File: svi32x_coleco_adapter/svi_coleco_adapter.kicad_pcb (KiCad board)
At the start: 2 copper layers, 212 x 94 mm, 62 parts, among them J1 Conn_01x09, J2 Conn_01x09, J3 COLECO cartridge slot, J4 SVI external bus connector, T1 NPN_BCE_9014B, T2 NPN_BCE_9014B, U1 74LS244, U10 27C64, U11 L79L05, U2 74LS244, U3 74LS32, U4 74LS00, U5 74LS00, U6 74LS138, U7 74LS138, U8 LM741, U9 SN76489

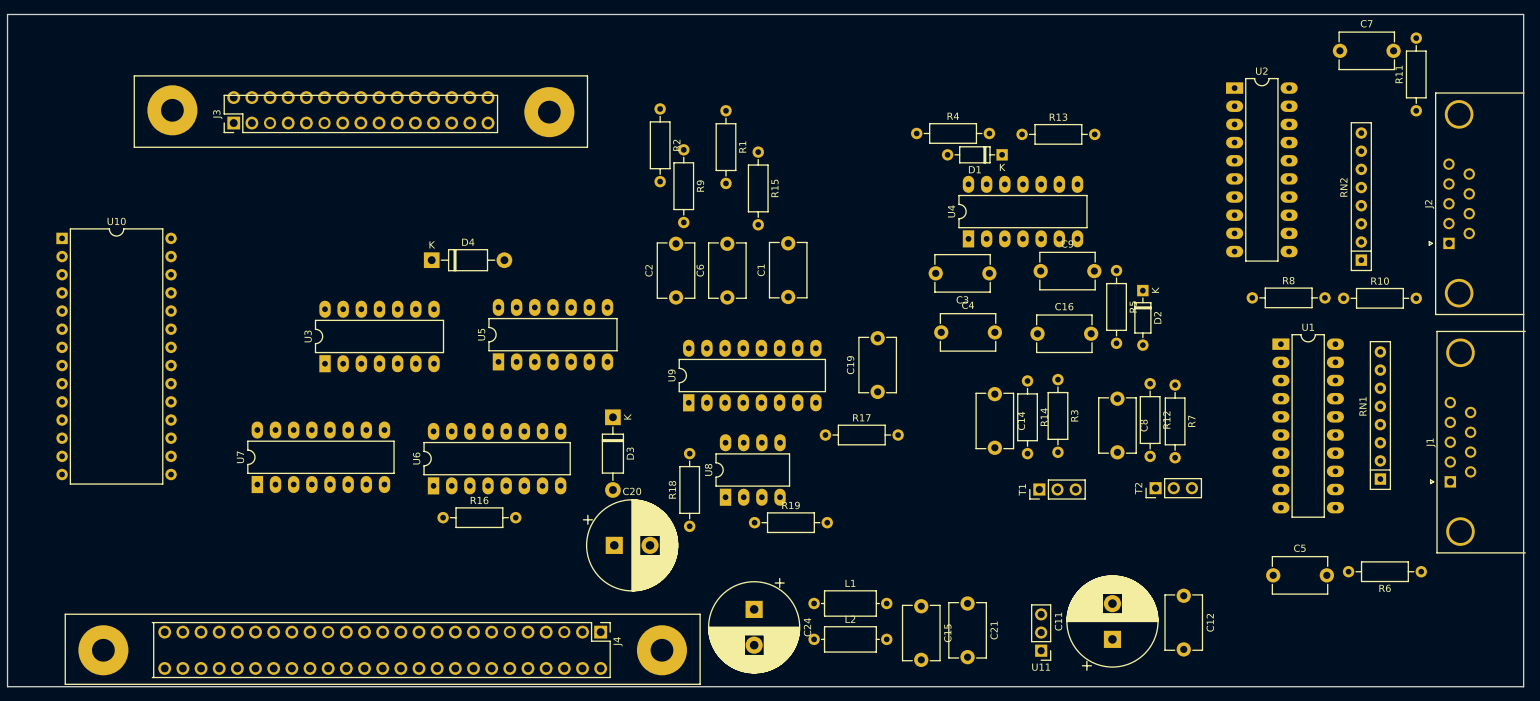
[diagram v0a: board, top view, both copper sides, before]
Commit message: Add files via upload
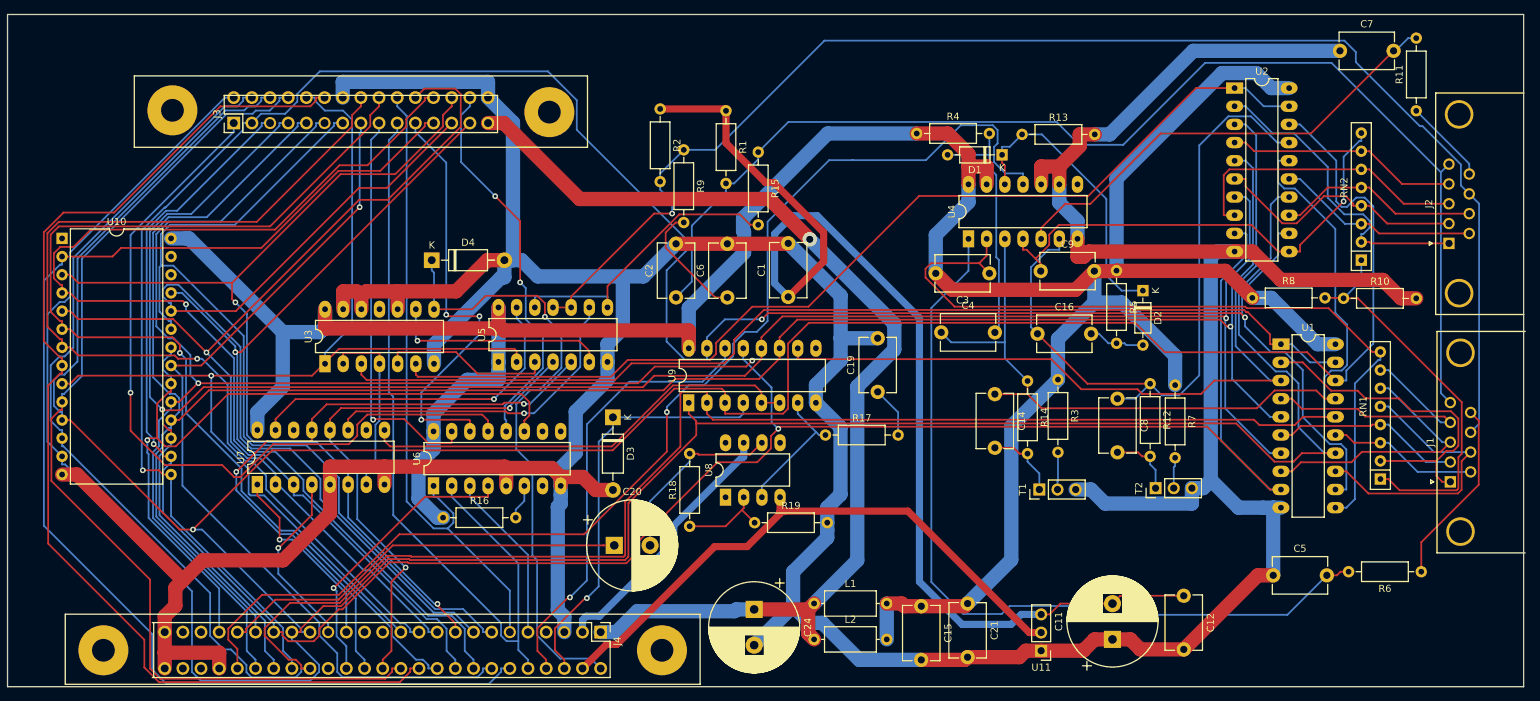
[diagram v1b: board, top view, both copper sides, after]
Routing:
- net GND: track 0.00 -> 662.8 mm
- net +5V: track 0.00 -> 420.1 mm
- net D1: track 0.00 -> 348.3 mm
- net D2: track 0.00 -> 343.8 mm
- net D0: track 0.00 -> 342.2 mm, vias 0 -> 1
- net D3: track 0.00 -> 321.8 mm, vias 0 -> 3
- net D4: track 0.00 -> 305.8 mm, vias 0 -> 2
- net D7: track 0.00 -> 304.5 mm, vias 0 -> 2
- net D5: track 0.00 -> 294.9 mm, vias 0 -> 2
- net D6: track 0.00 -> 292.1 mm, vias 0 -> 1
- net COL_JOY8: track 0.00 -> 195.9 mm, vias 0 -> 1
- net A12: track 0.00 -> 177.2 mm
- net COL_JOY5: track 0.00 -> 169.7 mm
- net _INT: track 0.00 -> 166.9 mm, vias 0 -> 1
- net A1: track 0.00 -> 159.0 mm, vias 0 -> 1
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
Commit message: Add files via upload
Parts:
- added C30: 100nf, Capacitor_THT:C_Disc_D7.0mm_W2.5mm_P5.00mm, F.Cu at (174.6, 36.1)
- added C31: 100nf, Capacitor_THT:C_Disc_D7.0mm_W2.5mm_P5.00mm, F.Cu at (196.5, 35.9)
- added C32: 100nf, Capacitor_THT:C_Disc_D7.0mm_W2.5mm_P5.00mm, F.Cu at (209.9, 91.8)
- added C33: 100nf, Capacitor_THT:C_Disc_D7.0mm_W2.5mm_P5.00mm, F.Cu at (229.2, 91.4)
- added C34: 100nf, Capacitor_THT:C_Disc_D7.0mm_W2.5mm_P5.00mm, F.Cu at (232.7, 34.7)
- added C35: 100nf, Capacitor_THT:C_Disc_D7.0mm_W2.5mm_P5.00mm, F.Cu at (256.6, 45.8)
- added C36: 100nf, Capacitor_THT:C_Disc_D7.0mm_W2.5mm_P5.00mm, F.Cu at (252.6, 115.3)
- added C37: 100nf, Capacitor_THT:C_Disc_D7.0mm_W2.5mm_P5.00mm, F.Cu at (79.6, 91.8)
- C1, C12, C14, C15, C16, C19, C2, C21, C3, C4, C5, C6, C7, C8, C9: footprint Capacitor_THT:C_Disc_D7.5mm_W5.0mm_P7.50mm -> Capacitor_THT:C_Disc_D7.0mm_W2.5mm_P5.00mm
- C20: footprint Capacitor_THT:CP_Radial_D12.5mm_P5.00mm -> Capacitor_THT:CP_Radial_D8.0mm_P5.00mm
- R12, R14: value 22R -> 22K
- moved R9 151.3 mm to (291.5, 77.7), turned to 180 degrees
- moved R2 145.0 mm to (281.3, 74.4), turned to 0 degrees
- moved U3 144.8 mm to (237.0, 88.1), turned to 180 degrees
- moved C2 136.3 mm to (276.6, 89.2), turned to 180 degrees
- moved C6 133.2 mm to (281.5, 80.9), turned to 0 degrees
- moved R1 131.7 mm to (276.5, 76.2)
- moved R15 125.0 mm to (273.6, 84.0), turned to 180 degrees
- moved J3 121.3 mm to (181.4, 113.2)
- moved C1 119.6 mm to (276.8, 73.4), turned to 180 degrees
- moved R16 109.7 mm to (209.0, 57.7), turned to 90 degrees
- moved U7 105.8 mm to (180.7, 57.4), turned to 180 degrees
- moved C15 105.1 mm to (85.0, 61.7), turned to 90 degrees
- moved L2 104.7 mm to (70.5, 61.3)
- moved U6 103.3 mm to (202.6, 57.4), turned to 180 degrees
- moved U5 101.4 mm to (217.7, 88.4), turned to 180 degrees
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- renumbered L2 to L1, L1 to L2
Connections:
- C21 pad 1: +5V -> 5V_COL
- J3 pad 30: 5V -> 5V_COL
- L1 pad 2: +5V -> 5V_COL
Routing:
- net GND: track 662.8 -> 824.5 mm, vias 0 -> 1
- net _MREQ: track 40.4 -> 194.1 mm
- net _EXCSR: track 75.3 -> 225.4 mm
- net _CNTRL2: track 86.5 -> 221.9 mm
- net COL_JOY5: track 169.7 -> 49.6 mm
- net MINUS12V: track 82.5 -> 201.8 mm
- net _IORQ: track 25.5 -> 137.7 mm, vias 1 -> 2
- net _WR: track 26.9 -> 138.6 mm
- net J2_ENABLE: track 142.4 -> 32.3 mm
- net A15: track 23.8 -> 132.4 mm, vias 0 -> 1
- net _EXCSW: track 91.0 -> 195.3 mm, vias 2 -> 3
- net J1_ENABLE: track 147.1 -> 45.9 mm
- net _WAIT: track 59.1 -> 157.7 mm, vias 1 -> 2
- net A7: track 134.5 -> 232.4 mm, vias 2 -> 1
- net +5V: track 420.1 -> 508.2 mm
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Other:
- board size 212 x 94 mm -> 250 x 100 mm
